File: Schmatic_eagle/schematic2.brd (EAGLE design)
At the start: 100 x 80 mm, 15 parts, among them IC1 MEGA16-A, IC2 MC145027DW, M1 WIRELESS-XY-MK-5V

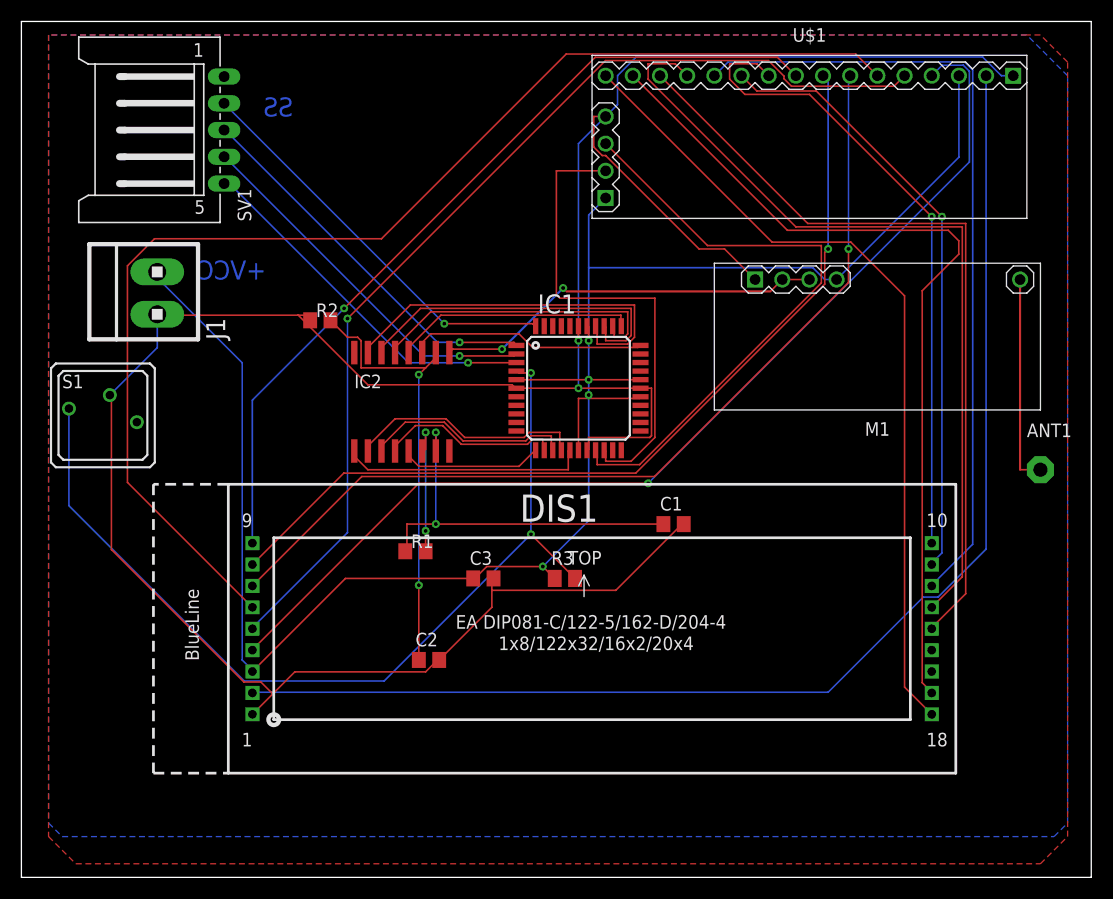
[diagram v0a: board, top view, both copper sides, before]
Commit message: Schematic 2 updates
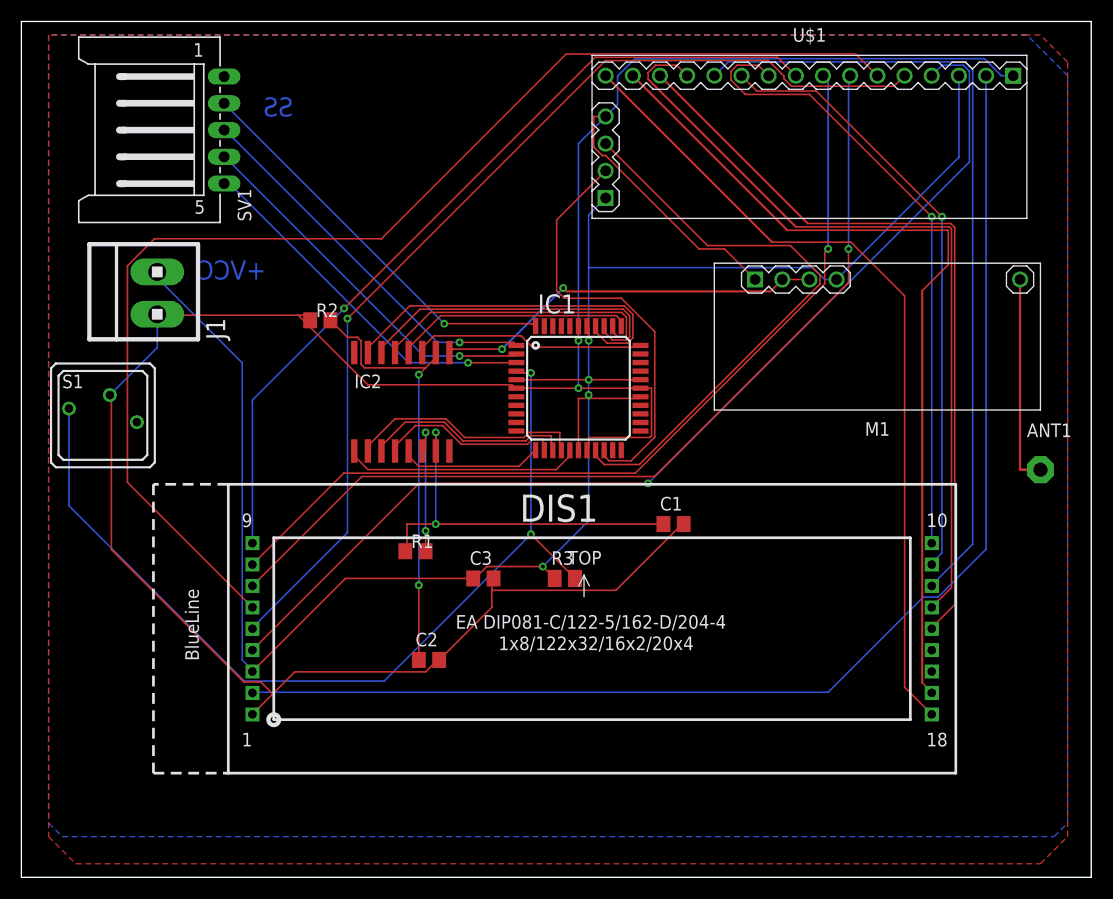
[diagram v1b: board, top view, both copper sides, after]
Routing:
- net N$22: track 45.2 -> 40.1 mm
- net N$21: track 57.0 -> 54.8 mm
- net N$34: track 77.4 -> 75.2 mm
- net N$38: track 73.5 -> 71.8 mm
- net N$7: track 35.6 -> 34.0 mm
- net N$8: track 31.9 -> 30.7 mm
- net N$6: track 28.2 -> 27.4 mm
- net N$36: track 80.9 -> 80.1 mm
- net N$1: track 22.9 -> 22.2 mm
- net N$30: track 60.3 -> 59.5 mm
